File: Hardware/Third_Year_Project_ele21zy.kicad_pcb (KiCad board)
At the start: 2 copper layers, 40 x 60 mm, 8 parts, among them J1 826926-5, J2 826926-5, J3 826926-5, J4 826926-5, J5 826926-5, J6 501876-2640

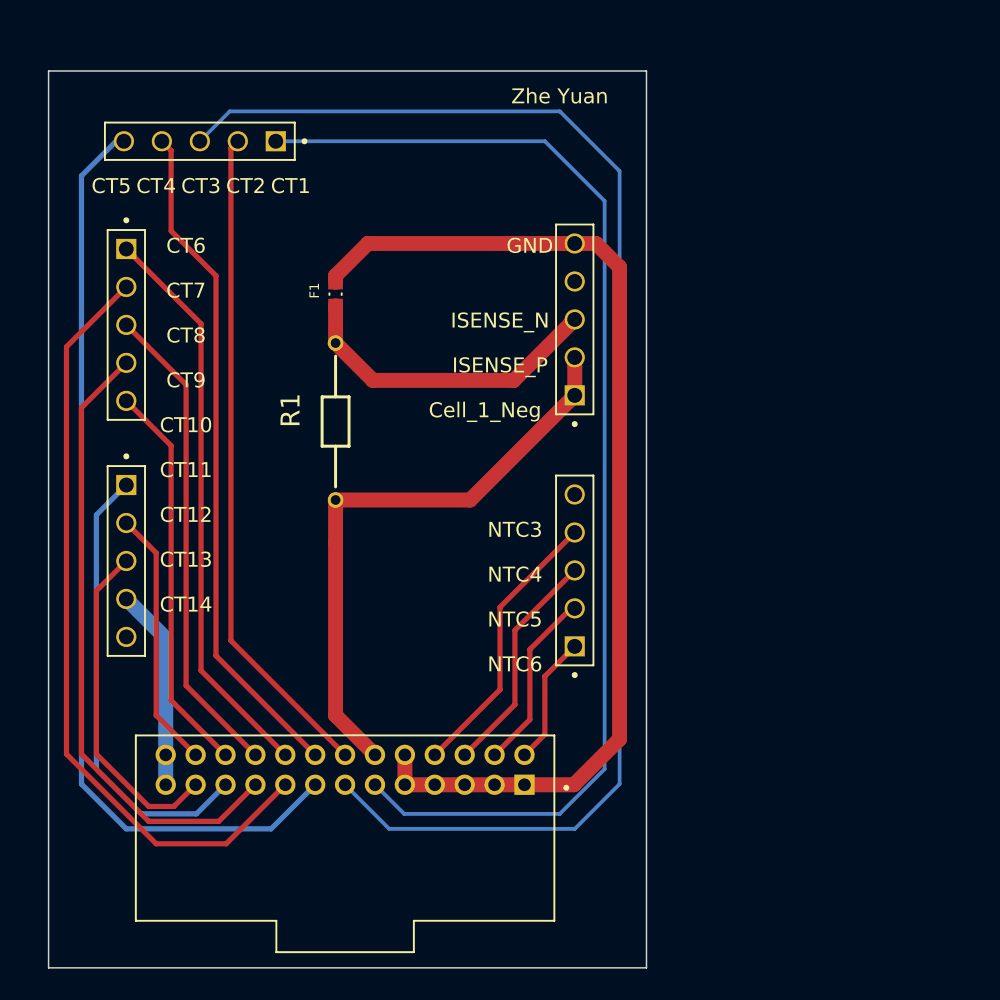
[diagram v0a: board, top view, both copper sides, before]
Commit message: update hardware
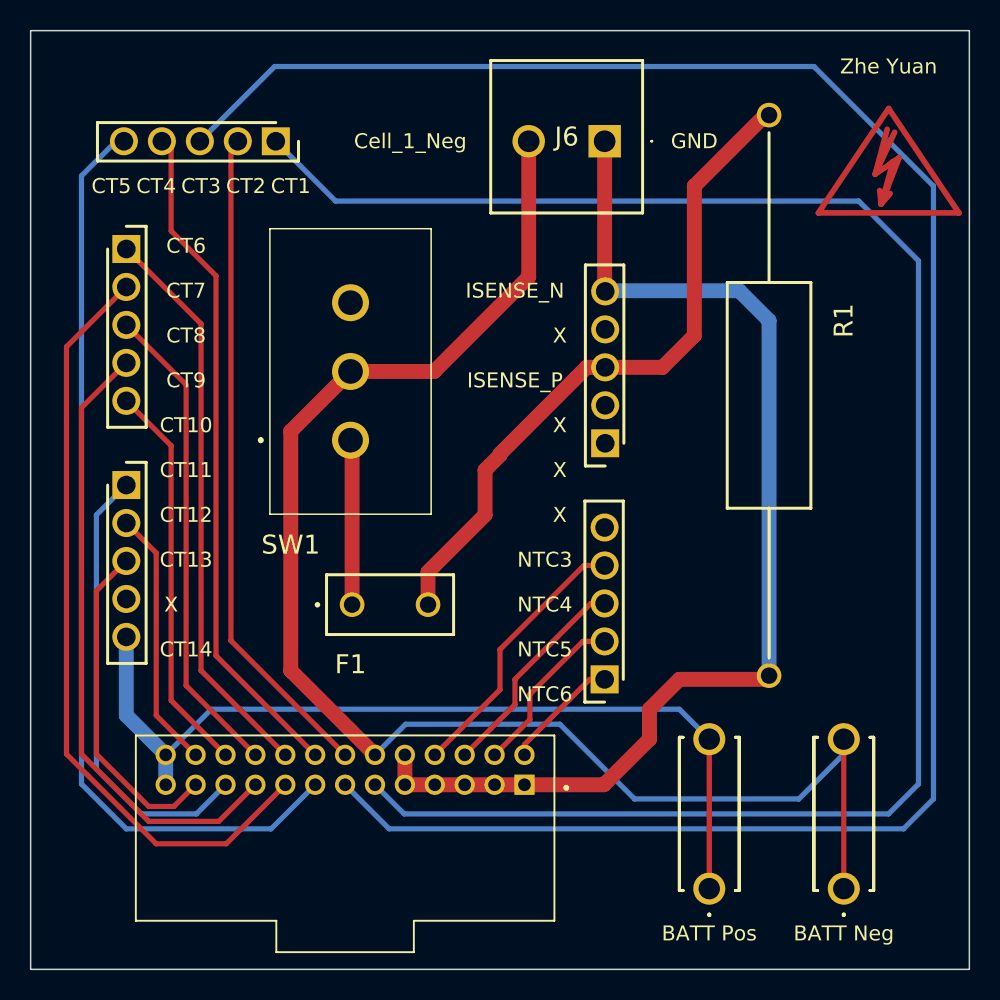
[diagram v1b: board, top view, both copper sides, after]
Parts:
- added J6: MC000048, MC000048:MC000048, F.Cu at (161.0, 72.0)
- added REF**: Symbol_HighVoltage_Type2_CopperTop_VerySmall, Symbol:Symbol_HighVoltage_Type2_CopperTop_VerySmall, F.Cu at (180.0, 74.0)
- added SW1: L102011MS02Q, L102011MS02Q:L102011MS02Q, F.Cu at (144.0, 92.0)
- added TP1: 930224100, 930224100:930224100, F.Cu at (168.0, 122.0)
- added TP2: 930224100, 930224100:930224100, F.Cu at (177.0, 122.0)
- F1: value 0686F2000-01 -> 39212000440; footprint 0686F2000-01:FUSC1608X60N -> 39212000440:39213150440_1
- J1, J2, J3, J4, J5: footprint 826926-5:TE_826926-5 -> 2212S-05SG-85:RHDR5W74P0X254_1X5_1320X250X850P
- R1: value 0.1 -> 43FR10E; footprint KiCad:RESAD1050W45L330D180 -> 43FR10E:RESAD3750W90L1510D560
- moved R1 38.8 mm to (172.0, 70.2), turned to -90 degrees
- moved F1 21.1 mm to (146.6, 103.0), turned to 0 degrees
- moved J5 3.80 mm to (161.0, 92.2)
- moved J1 2.98 mm to (161.0, 108.0)
- renumbered J6 to J7
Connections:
- F1 pad 1: ISENSE_N -> Net-(F1-Pad1)
- F1 pad 2: GND -> ISENSE_P
- J4 pad 4: CELL_14 -> unconnected-(J4-Pad4)
- J4 pad 5: unconnected-(J4-Pad5) -> CELL_14
- J5 pad 1: CELL_1_Negative -> unconnected-(J5-Pad1)
- J5 pad 2: CELL_1_Negative -> unconnected-(J5-Pad2)
- J5 pad 3: ISENSE_N -> ISENSE_P
- R1 pad 1: CELL_1_Negative -> ISENSE_P
- R1 pad 2: ISENSE_N -> GND
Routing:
- net CELL_1_Negative: track 39.6 -> 99.5 mm
- net CELL_14: track 13.5 -> 59.4 mm
- net ISENSE_P: track 0.00 -> 45.3 mm
- net CELL_3: track 92.4 -> 136.9 mm
- net CELL_1: track 79.1 -> 119.3 mm
- net ISENSE_N: track 21.2 -> 0.00 mm
- net Net-(F1-Pad1): track 0.00 -> 11.0 mm
- net GND: track 70.2 -> 75.9 mm
- net NTC4: track 15.4 -> 14.5 mm
- net NTC6: track 8.65 -> 7.86 mm
- net NTC5: track 12.2 -> 11.5 mm
- net NTC3: track 18.8 -> 18.2 mm
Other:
- board size 40 x 60 mm -> 62.8 x 62.8 mm
- board text added: "BATT Neg"
- board text added: "BATT Pos"
- board text added: "X"
